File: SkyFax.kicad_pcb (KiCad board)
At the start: 2 copper layers, 60 parts, among them J1 RJ11/12, J2 DE9_Receptacle_MountingHoles, Q1 Q_NPN_BEC, Q2 Q_PNP_BEC, Q3 Q_NPN_BEC, Q4 Q_NPN_BEC, Q5 Q_NPN_BEC, Q6 Q_NPN_EBC, SW1 SW_DIP_x08, U1 Si2494-A-FM, U2 Si3018, U3 25LC640AT-E/SN, X1 ECS-2520MV-xxx-xx

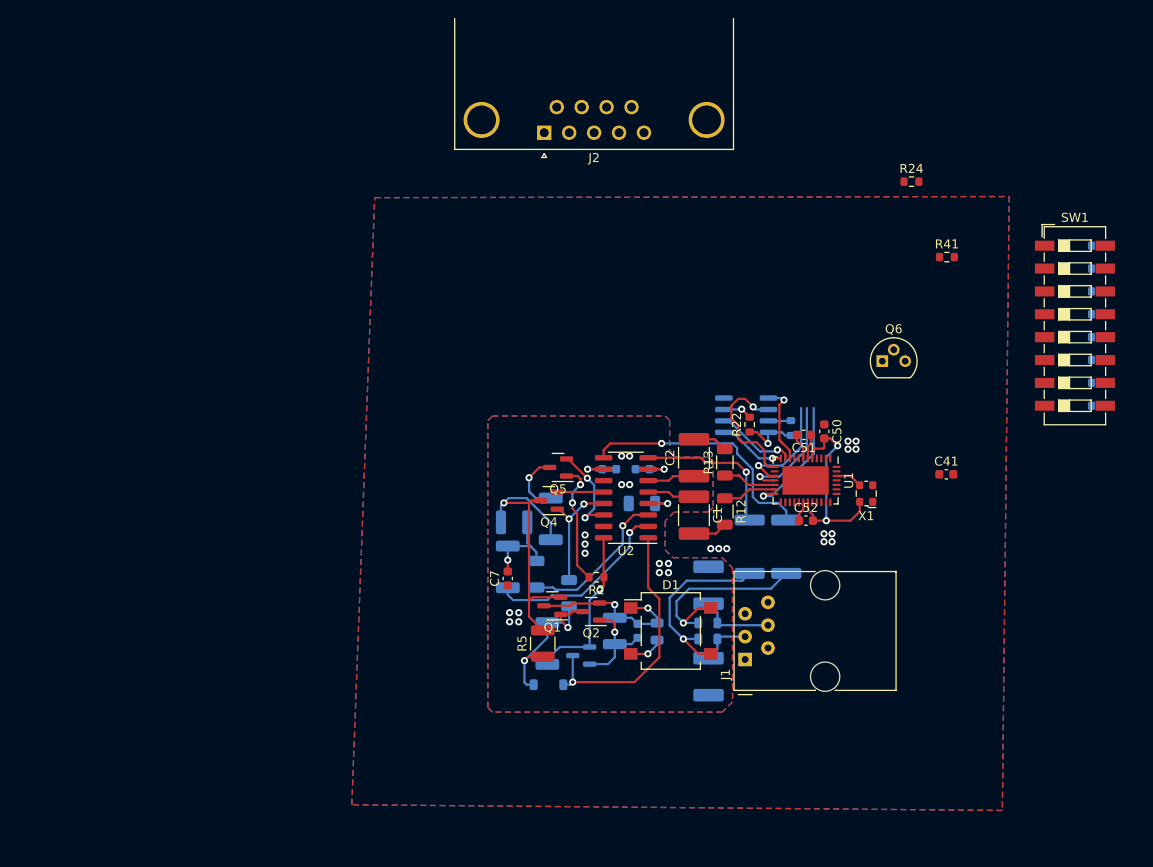
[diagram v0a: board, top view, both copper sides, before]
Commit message: Sent to fab v1.0
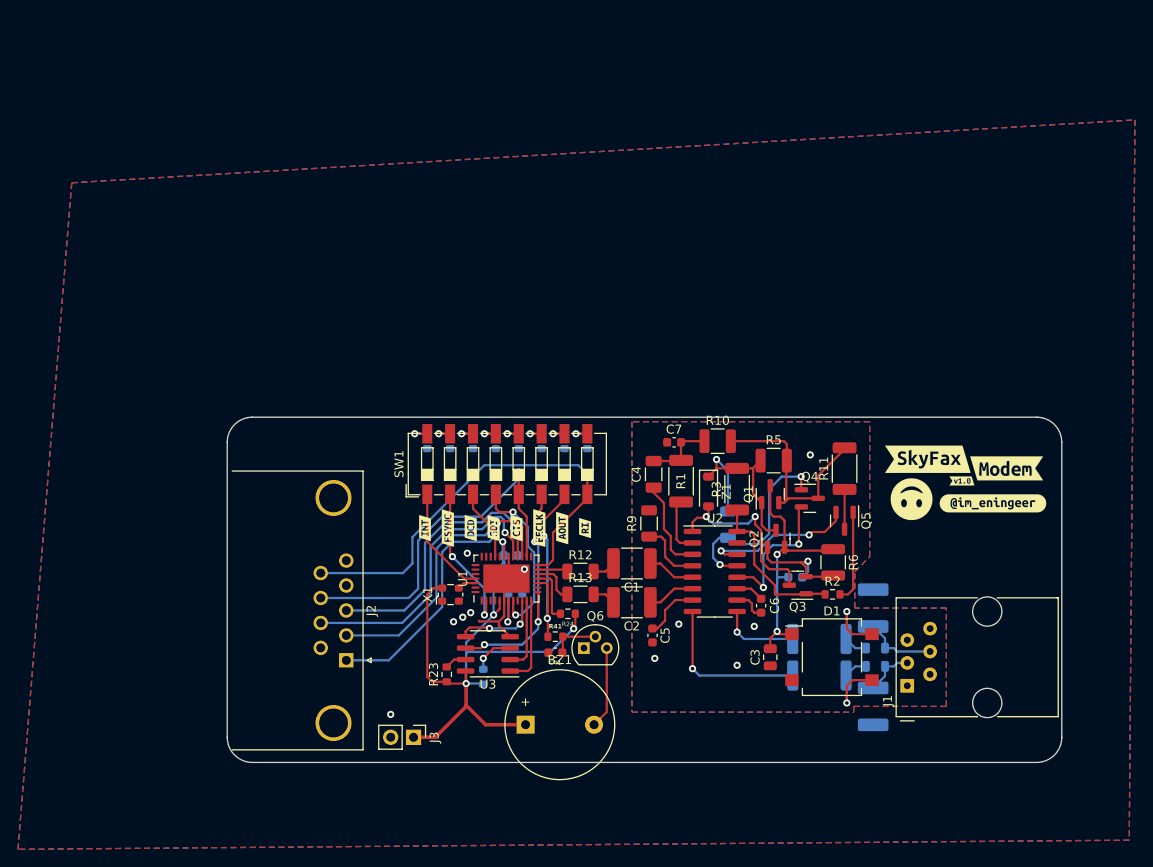
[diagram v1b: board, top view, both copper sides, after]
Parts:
- removed kibuzzard-649E5FCF: G***, kibuzzard-649E5FCF
- removed kibuzzard-649E606C: G***, kibuzzard-649E606C
- removed kibuzzard-649E607D: G***, kibuzzard-649E607D
- removed kibuzzard-649E6159: G***, kibuzzard-649E6159
- added BZ1: Buzzer, Buzzer_Beeper:Buzzer_12x9.5RM7.6, F.Cu at (108.2, 146.6)
- added G***: LOGO, FaxCam:smiley_5.0x5.2mm, F.Cu at (151.1, 121.6)
- added J3: Conn_01x02, Connector_PinHeader_2.54mm:PinHeader_1x02_P2.54mm_Vertical, F.Cu at (95.8, 148.0)
- added kibuzzard-64A46BC3: G***, kibuzzard-64A46BC3, F.Cu at (161.6, 118.1)
- added kibuzzard-64A46BC7: G***, kibuzzard-64A46BC7, F.Cu at (152.9, 117.1)
- added kibuzzard-64A46BF2: G***, kibuzzard-64A46BF2, F.Cu at (156.7, 119.5)
- added kibuzzard-64A46C0A: G***, kibuzzard-64A46C0A, F.Cu at (160.1, 122.0)
- added kibuzzard-64A46CB2: G***, kibuzzard-64A46CB2, F.Cu at (97.0, 124.7)
- added kibuzzard-64A46CE2: G***, kibuzzard-64A46CE2, F.Cu at (99.6, 124.7)
- added kibuzzard-64A46CEC: G***, kibuzzard-64A46CEC, F.Cu at (102.1, 124.7)
- added kibuzzard-64A46CF4: G***, kibuzzard-64A46CF4, F.Cu at (104.6, 124.7)
- added kibuzzard-64A46CF9: G***, kibuzzard-64A46CF9, F.Cu at (107.2, 124.7)
- added kibuzzard-64A46D01: G***, kibuzzard-64A46D01, F.Cu at (109.7, 124.7)
- added kibuzzard-64A46D0F: G***, kibuzzard-64A46D0F, F.Cu at (112.3, 124.7)
- added kibuzzard-64A46D1C: G***, kibuzzard-64A46D1C, F.Cu at (114.8, 124.7)
- C3, C4, C5, C6, Q3, R1, R10, R11, R23, R3, R6, R9, U3, Z1: moved to F.Cu
- C50, C51, C52, R22: moved to B.Cu
- moved R14 77.7 mm to (97.3, 115.1), turned to -90 degrees
- moved R15 74.6 mm to (99.8, 115.1), turned to -90 degrees
- moved R16 71.5 mm to (102.4, 115.1), turned to -90 degrees
- moved R17 68.5 mm to (104.9, 115.1), turned to -90 degrees
- moved R18 65.5 mm to (107.4, 115.1), turned to -90 degrees
- moved SW1 64.9 mm to (106.2, 117.6), turned to 90 degrees
- moved J2 62.6 mm to (88.3, 139.4), turned to -90 degrees
- moved R19 62.6 mm to (110.0, 115.1), turned to -90 degrees
- moved R24 61.3 mm to (112.9, 134.2), turned to 180 degrees
- moved R41 60.6 mm to (111.5, 136.8), turned to 180 degrees
- moved R20 59.7 mm to (112.5, 115.1), turned to -90 degrees
- moved R21 57.0 mm to (115.1, 115.1), turned to -90 degrees
- moved C41 47.7 mm to (111.5, 138.6), turned to 180 degrees
- moved X1 47.5 mm to (99.9, 132.1), turned to 90 degrees
- moved R23 47.0 mm to (99.4, 141.0)
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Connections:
- SW1 pad 1: /nFSYNC -> /nINT
- SW1 pad 2: /nCTS -> /nFSYNC
- SW1 pad 3: /SDI -> /nDCD
- SW1 pad 4: /AOUT -> /SDI
- SW1 pad 5: /EECLK -> /nCTS
- SW1 pad 6: /nINT -> /EECLK
- SW1 pad 7: /nRI -> /AOUT
- SW1 pad 8: /nDCD -> /nRI
- U1 pad 39: (no net) -> GND
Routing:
- net +3V3: track 29.4 -> 72.4 mm, vias 3 -> 4
- net /nCTS: track 0.00 -> 41.1 mm, vias 0 -> 1
- net /nRI: track 14.0 -> 49.8 mm
- net /nDCD: track 0.00 -> 33.8 mm, vias 0 -> 1
- net /nRTS: track 0.00 -> 33.0 mm, vias 0 -> 1
- net /RXD: track 0.00 -> 31.6 mm, vias 0 -> 1
- net /TXD: track 0.00 -> 30.5 mm, vias 0 -> 1
- net /SDI: track 0.00 -> 19.0 mm, vias 0 -> 2
- net Net-(U2-RNG2): track 27.7 -> 8.78 mm
- net /nFSYNC: track 0.00 -> 16.7 mm, vias 0 -> 2
- net Net-(U2-DCT): track 21.0 -> 6.31 mm, vias 1 -> 0
- net /EECLK: track 15.1 -> 27.7 mm, vias 1 -> 3
- net /nINT: track 0.00 -> 12.3 mm
- net Net-(D1-Pad4): track 21.6 -> 10.7 mm
- net Net-(Q4-E): track 5.14 -> 15.7 mm, vias 0 -> 2
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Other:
- board outline added: 92.7 x 38.4 mm
